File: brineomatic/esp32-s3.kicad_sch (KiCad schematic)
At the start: 27 parts, among them J19 USB_TYPE_C_16PIN, SW1 RESET, SW2 BOOT, U5 ESP32-S3-WROOM-1-N16R8, U6 USBLC6-2SC6, U7 SN74LV1T34DBV, U8 XC6210B332MR

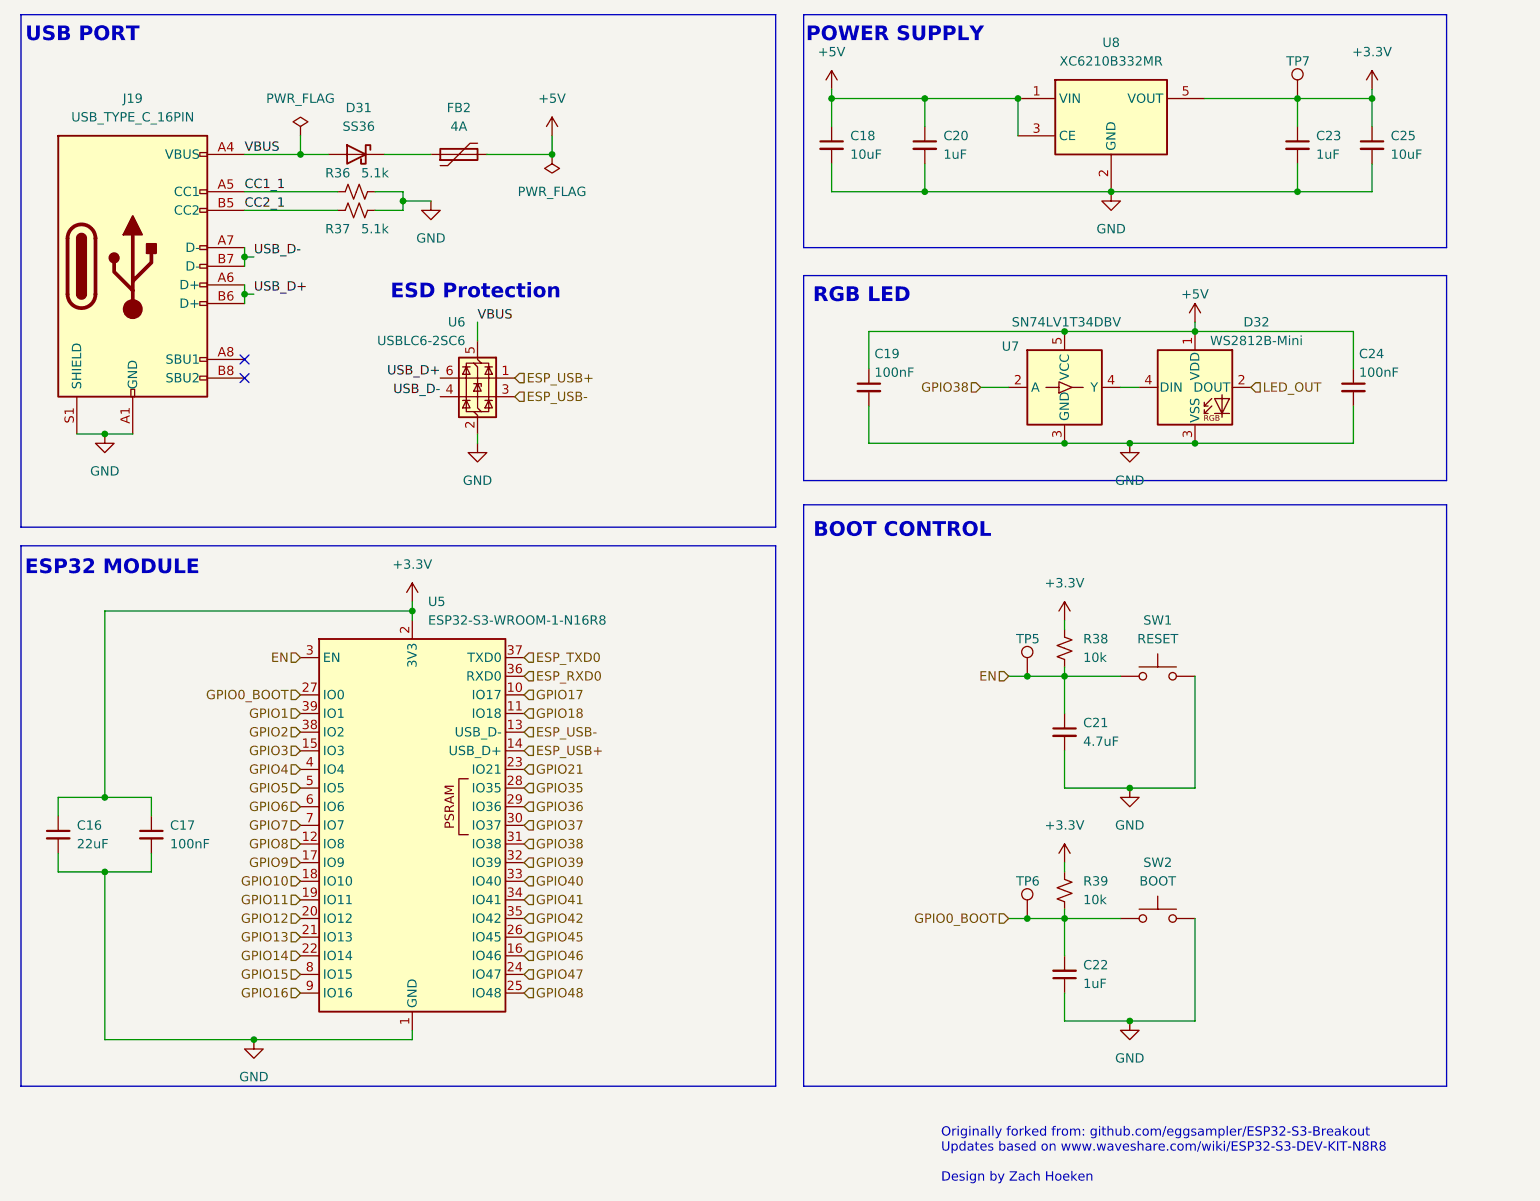
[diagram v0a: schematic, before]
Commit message: small cleanups on schematic
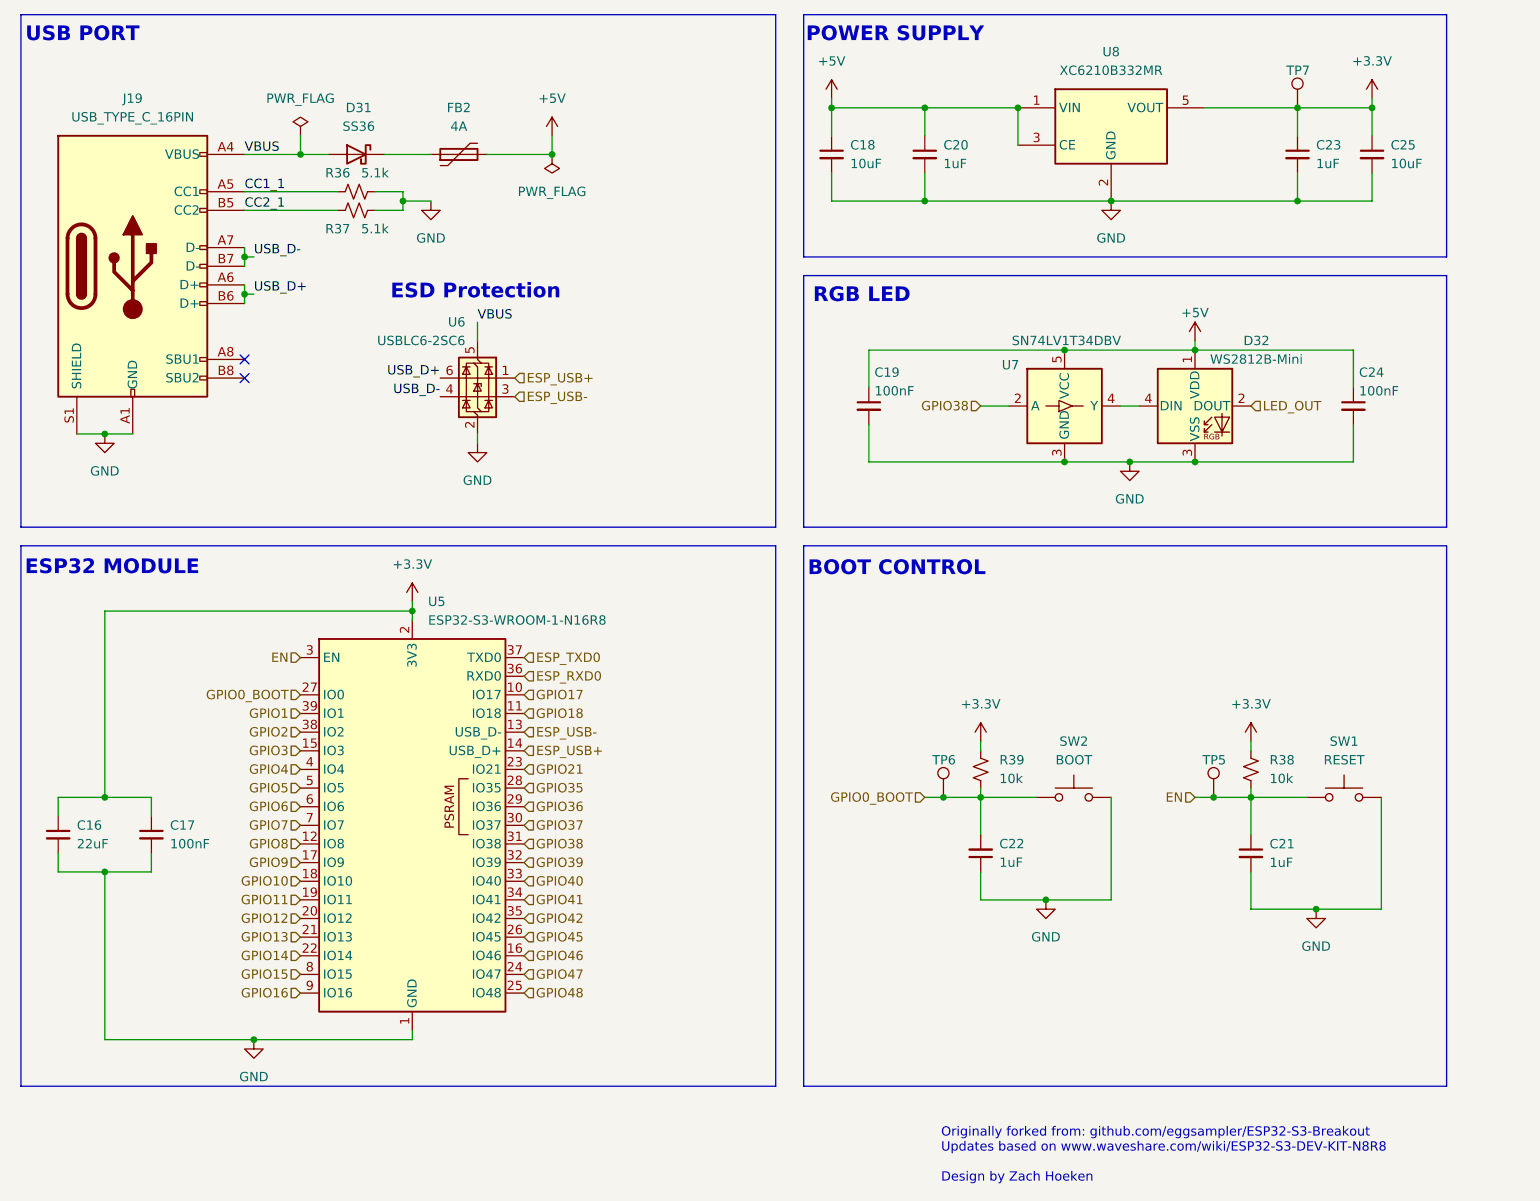
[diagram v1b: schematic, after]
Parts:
- C21: value 4.7uF -> 1uF
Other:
- moved on the sheet: C18, C19, C20, C21, C22, C23, C24, C25, D32, R38, R39, SW1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
